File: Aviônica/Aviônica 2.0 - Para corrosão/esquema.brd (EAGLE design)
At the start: 129 x 66 mm, 15 parts, among them M1 WIRELESS-NRF24L01-PA-EXT

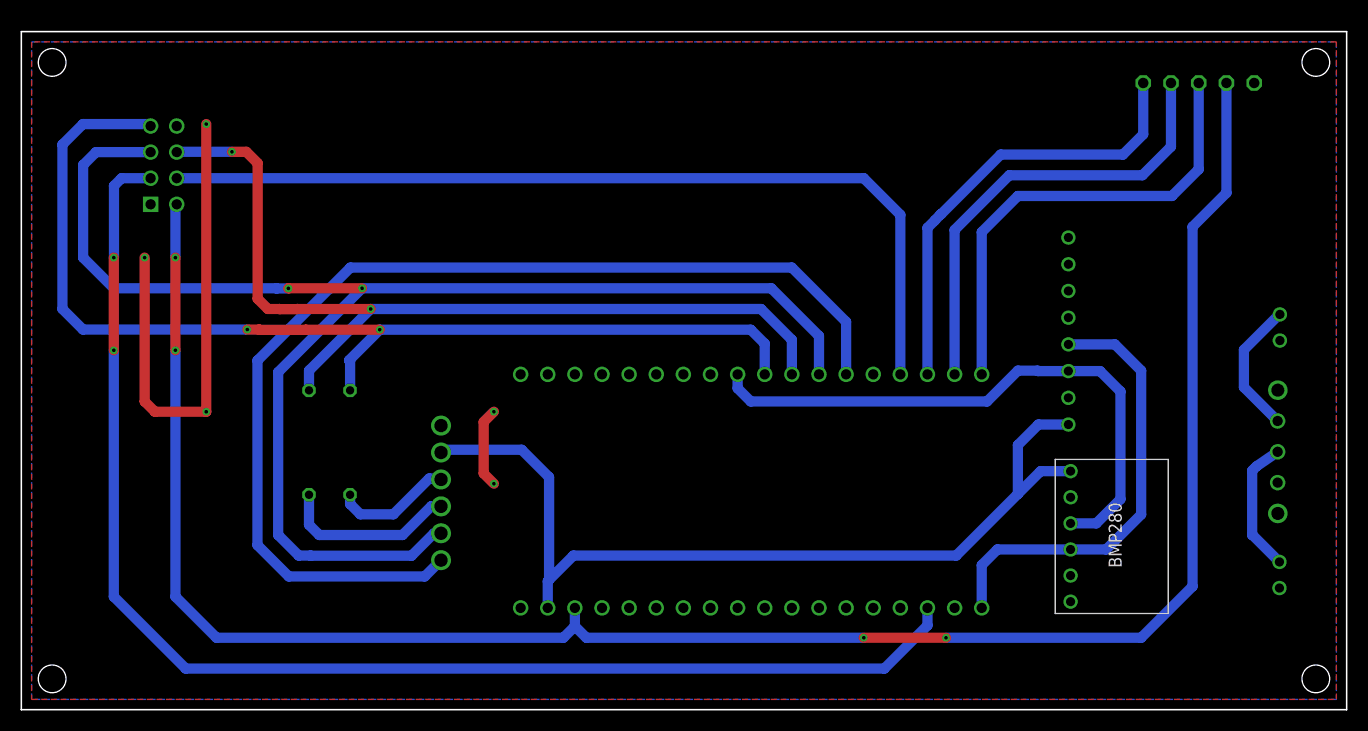
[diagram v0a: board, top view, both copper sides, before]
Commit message: Update
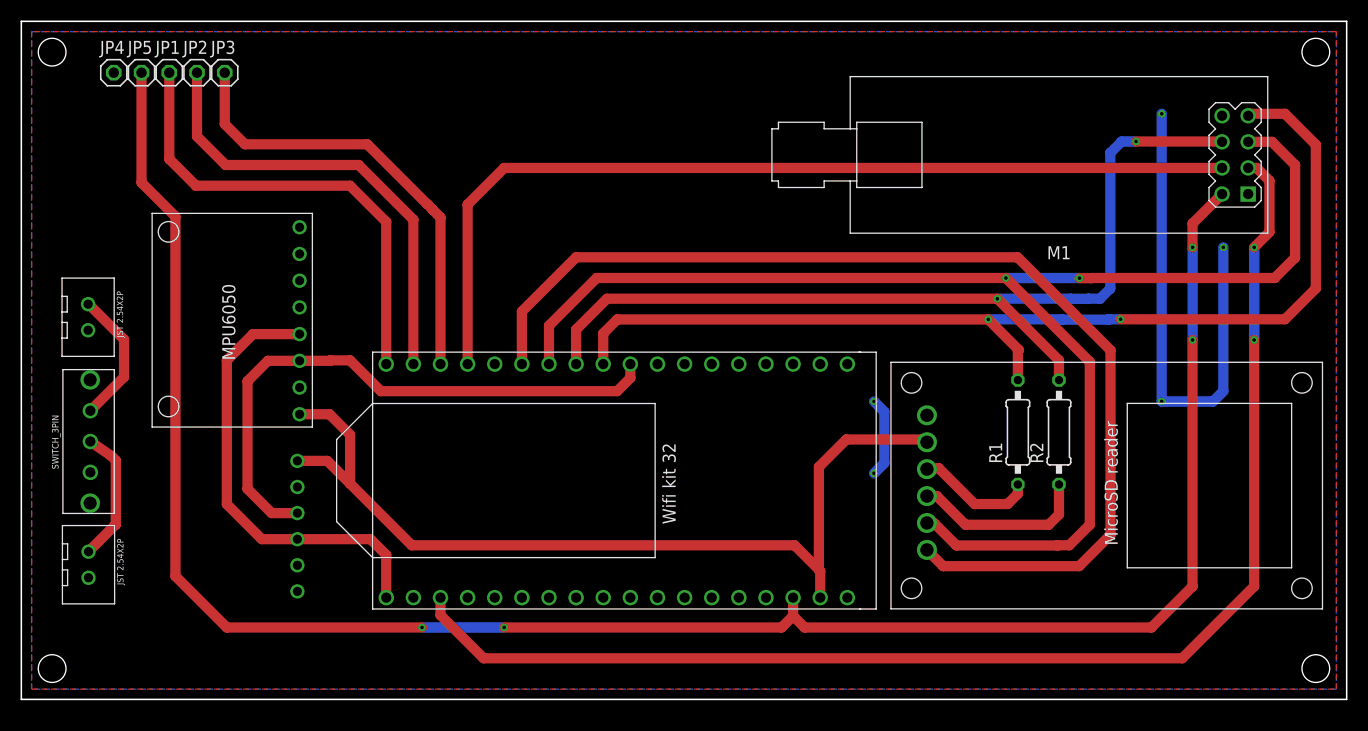
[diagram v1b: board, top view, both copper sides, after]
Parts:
- moved U$7 116.0 mm to (6.50, 34.2), flipped to the top
- moved U$5 115.9 mm to (6.54, 10.1), flipped to the top
- moved U$6 115.6 mm to (6.70, 22.1), flipped to the top
- moved JP4 111.0 mm to (9.00, 58.0), flipped to the top
- moved JP5 105.6 mm to (11.7, 58.0), flipped to the top
- moved JP1 100.2 mm to (14.4, 58.0), flipped to the top
- moved U$3 95.2 mm to (16.9, 33.7), flipped to the top
- moved JP2 94.8 mm to (17.1, 58.0), flipped to the top
- moved JP3 89.4 mm to (19.8, 58.0), flipped to the top
- moved U$1 87.5 mm to (20.8, 13.7), flipped to the bottom
- moved R2 73.0 mm to (101.0, 23.0), flipped to the top
- moved M1 70.0 mm to (101.0, 50.0), flipped to the top
- moved R1 65.0 mm to (97.0, 23.0), flipped to the top
- moved U$2 64.7 mm to (96.8, 18.0), flipped to the top
- moved U$4 5.49 mm to (67.2, 18.3), flipped to the top
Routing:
- net CSN_NRF: track 87.4 -> 90.4 mm
- net MOSI: track 89.0 -> 92.0 mm
- net MISO: track 105.4 -> 103.3 mm
- net CE: track 129.4 -> 128.2 mm
- net 3V3_2: track 194.0 -> 195.2 mm
- net SCLK: track 139.6 -> 138.6 mm
